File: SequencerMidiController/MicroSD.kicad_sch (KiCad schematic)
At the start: 1 part, among them J3 Conn_01x06

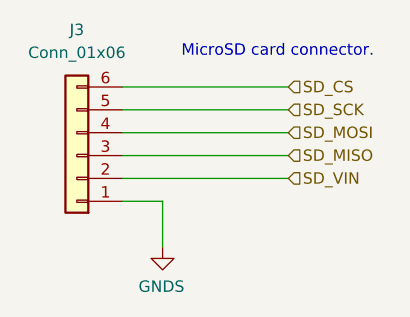
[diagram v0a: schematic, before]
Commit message: updated save
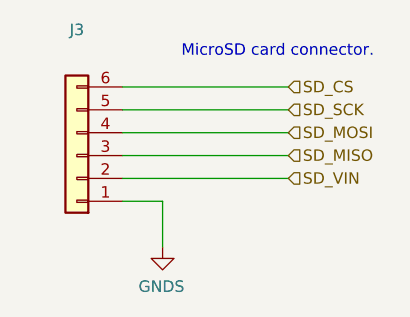
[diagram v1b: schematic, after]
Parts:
- J3: value Conn_01x06 -> (none); footprint Connector_PinSocket_2.54mm:PinSocket_1x06_P2.54mm_Horizontal -> (none)
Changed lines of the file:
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@@
     (in_bom yes) (on_board yes) (fields_autoplaced)
     (property "Reference" "J3" (id 0) (at 125.73 75.565 0))
-    (property "Value" "Conn_01x06" (id 1) (at 125.73 78.105 0))
-    (property "Footprint" "Connector_PinSocket_2.54mm:PinSocket_1x06_P2.54mm_Horizontal" (id 2) (at 125.73 89.535 0)
+    (property "Value" "" (id 1) (at 125.73 78.105 0))
+    (property "Footprint" "" (id 2) (at 125.73 89.535 0)
       (effects (font (size 1.27 1.27)) hide)
     )

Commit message: RevB
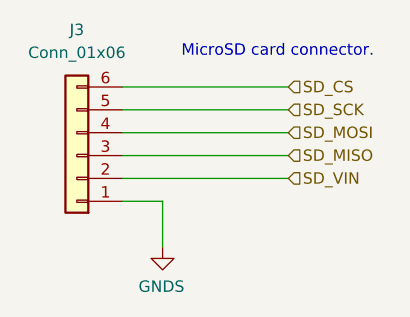
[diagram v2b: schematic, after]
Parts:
- J3: value (none) -> Conn_01x06; footprint (none) -> Connector_PinSocket_2.54mm:PinSocket_1x06_P2.54mm_Vertical
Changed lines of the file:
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@@
     (in_bom yes) (on_board yes) (fields_autoplaced)
     (property "Reference" "J3" (id 0) (at 125.73 75.565 0))
-    (property "Value" "" (id 1) (at 125.73 78.105 0))
-    (property "Footprint" "" (id 2) (at 125.73 89.535 0)
+    (property "Value" "Conn_01x06" (id 1) (at 125.73 78.105 0))
+    (property "Footprint" "Connector_PinSocket_2.54mm:PinSocket_1x06_P2.54mm_Vertical" (id 2) (at 125.73 89.535 0)
       (effects (font (size 1.27 1.27)) hide)
     )
